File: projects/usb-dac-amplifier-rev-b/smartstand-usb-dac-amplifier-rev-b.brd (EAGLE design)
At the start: 91 x 135.9 mm, 231 parts, among them J1 PJ-002A, J2 292304-1, J3 NRJ6HH, J4 PJRAN2X1U01AUX, J5 T1M-5POS, U1 XUF208-256-TQ64, U10 TPS3702, U11 PCM5102A, U12 SZNUD3124, U13 NJM2068M, U14 NJM4556AM, U15 NJM4556AM, U16 TS5A3159DBV, U17 SN74LVC3G34DCU, U18 TPD2E007DCK, U19 TPD2E007DCK, U2 TPD4E02B04DQA, U3 TPS563200DDC, U4 TPS7A8300RGW, U5 TPS563200DDC, U6 TPS7A8300RGW, U7 TPS7A8300RGW, U8 TPS7A4701RGW, U9 TPS7A3301RGW, X1 24MHz, X2 22.5792MHz, X3 24.576MHz

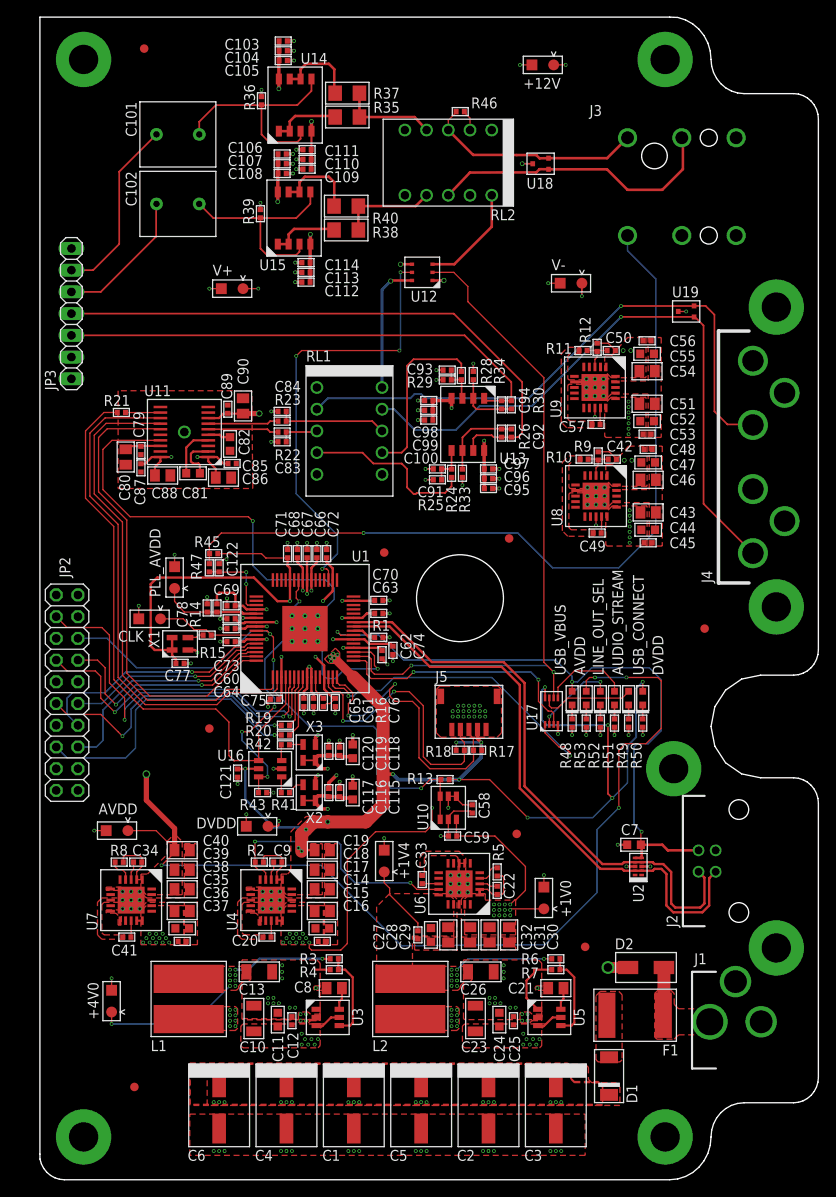
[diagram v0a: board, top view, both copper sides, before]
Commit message: Start attributizing things to help develop tooling.
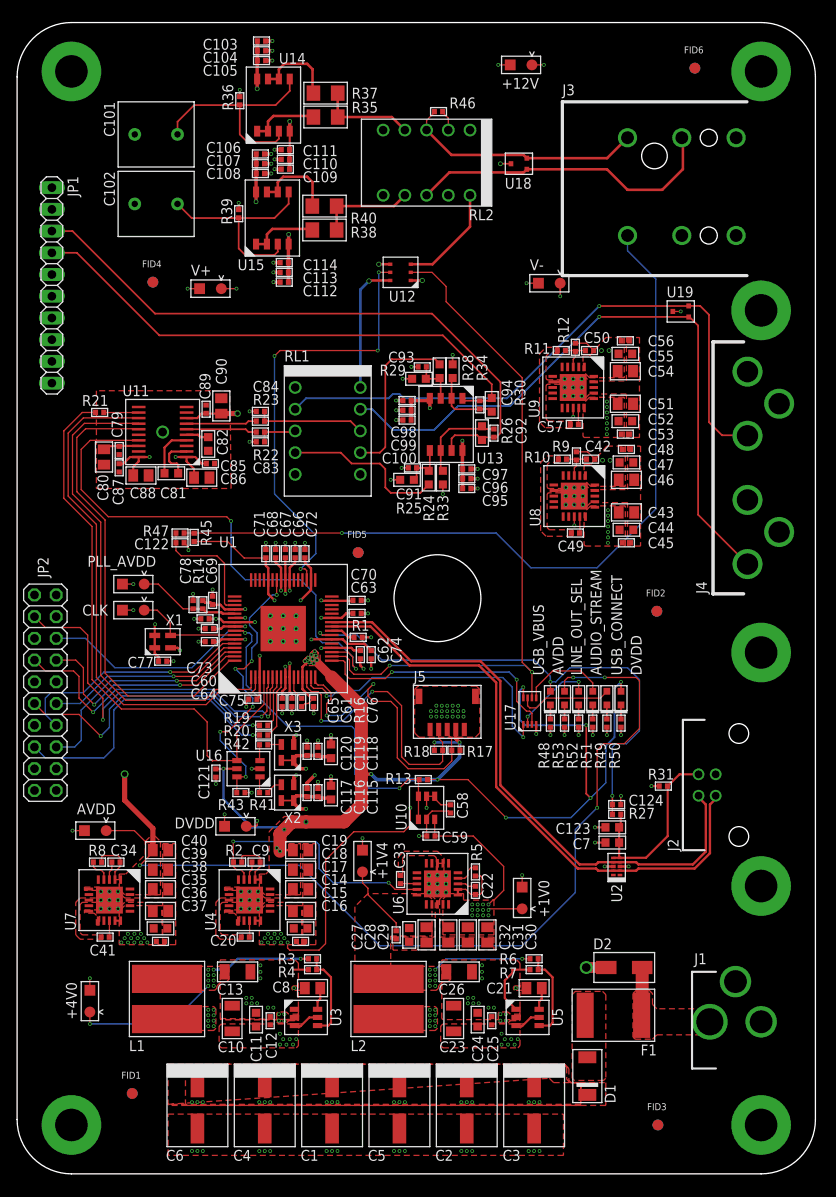
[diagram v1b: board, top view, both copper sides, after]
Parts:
- removed JP3: (no value), pin-headers:1X07
- removed R15: 0, rcl:R0402
- removed U$1, U$11, U$13, U$2, U$3, U$5, U$6, U$7: FIDUCIAL-1MM, fiducials:FIDUCIAL_1MM
- added C123: 1uF, passives:C0603
- added C124: 0.1uF, passives:C0402
- added FID1, FID2, FID3, FID4, FID5, FID6: FIDUCIAL_100MIL, MF_Aesthetics:FIDUCIAL_100MIL
- added JP1: (no value), pin-headers:1X10
- added R27: 10K, passives:R0402
- added R31: 18K, passives:R0402
- C10, C23: value 22uF -> 47uF
- C103, C106, C109, C112, C116, C119, C12, C121, C122, C16, C21, C25, C29, C37, C45, C48, C53, C56, C60, C61, C62, C63, C64, C65, C66, C67, C68, C69, C70, C71, C72, C73, C74, C75, C76, C77, C78, C79, C8, C85, C87, C89, C95, C98: value 100nF -> 0.1uF
- C104, C107, C110, C113, C117, C120, C20, C22, C33, C34, C41, C58, C59, C9, C96, C99: value 10nF -> 0.01uF
- C105, C108, C111, C114: value 33pF -> 27pF
- C42, C49, C50, C57: value 100nF -> 0.01uF
- L2: value 1.5uH -> 2.2uH
- R24, R28: value 243, 0.1% -> 270, 1%; device rcl:R0402 -> passives:R0603
- R25, R26, R29, R30: device rcl:R0402 -> passives:R0603
- R3: value 40.2K -> 40.2K, 1%
- R33, R34: value 715, 0.1% -> 1K, 0.1%; device rcl:R0402 -> passives:R0603
- R4, R7: value 10K -> 10K, 1%
- R46: value 10K, 0.1% -> 10K
- R49, R50, R51, R52, R53: value 150 -> 220
- R6: value 8.45K -> 9.53K, 1%
- U3, U5: value TPS563200DDC -> TPS563201DDC
- moved J2 8.89 mm to (89.3, -21.8)
- moved C122 5.43 mm to (19.1, 6.48), turned to 0 degrees
- moved R47 5.32 mm to (19.1, 7.62), turned to 180 degrees
- moved TP4 4.89 mm to (13.6, 1.65), turned to 180 degrees
- moved R25 3.56 mm to (45.6, 13.8)
- moved R29 3.30 mm to (47.0, 25.7)
- moved C73 3.05 mm to (22.0, -2.41)
- moved R45 2.98 mm to (20.7, 7.11), turned to 270 degrees
- moved C93 2.95 mm to (47.4, 27.1)
- moved C91 2.92 mm to (46.2, 15.2)
- moved R24 2.71 mm to (48.1, 14.1)
- moved C74 2.59 mm to (41.4, -6.60)
- moved R28 2.59 mm to (49.4, 26.5)
- moved C7 2.55 mm to (69.6, -28.6)
- moved C32 2.54 mm to (50.4, -39.4)
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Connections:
- removed net N$33: R15.1, X1.P$3
- new net N$231: C123.1, C7.1, J2.P$1, R27.1, R31.2, U2.P$5, U2.P$6
- net +12V: now also JP1.1; no longer JP3.1
- net ADJUSTED_LEFT: now also JP1.6; no longer JP3.6
- net ADJUSTED_RIGHT: now also JP1.5; no longer JP3.5
- net AGND: now also C123.2, C124.2, JP1.2, JP1.7, R31.1; no longer JP3.2, JP3.7
- net CLK: now also X1.P$3; no longer R15.2
- net DVDD: now also JP1.8
- net I2C_SCL: now also JP1.9
- net I2C_SDA: now also JP1.10
- net PREAMP_LEFT: now also JP1.3; no longer JP3.4
- net PREAMP_RIGHT: now also JP1.4; no longer JP3.3
- net USB_VBUS: now also C124.1, R27.2; no longer C7.1, J2.P$1, U2.P$5, U2.P$6
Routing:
- net DVDD: track 301.6 -> 275.7 mm, vias 30 -> 35
- net N$231: track 0.00 -> 22.7 mm
- net USB_VBUS: track 76.2 -> 62.8 mm
- net ADJUSTED_LEFT: track 21.5 -> 28.8 mm
- net AUDIO_ENABLE: track 68.8 -> 63.4 mm
- net JACK_DETECT: track 9.26 -> 14.4 mm, vias 2 -> 0
- net USB_CONNECTED: track 39.4 -> 34.5 mm
- net +1V0: track 113.7 -> 108.8 mm, vias 22 -> 23
- net PREAMP_LEFT: track 69.6 -> 73.6 mm
- net AGND: track 109.6 -> 113.6 mm, vias 146 -> 149
- net PREAMP_RIGHT: track 59.2 -> 63.1 mm
- net LINE_OUT_RIGHT: track 73.5 -> 76.7 mm
- net LINE_OUT_LEFT: track 68.8 -> 72.0 mm
- net N$27: track 25.8 -> 28.4 mm
- net N$29: track 34.4 -> 36.9 mm
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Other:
- board size 91 x 135.9 mm -> 93.3 x 134.6 mm
